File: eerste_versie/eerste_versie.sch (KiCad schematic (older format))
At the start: 16 parts, among them U1 ESP32-WROOM-32U, U2 AMS1117-3.3, X1 DG3XX-02-5.0

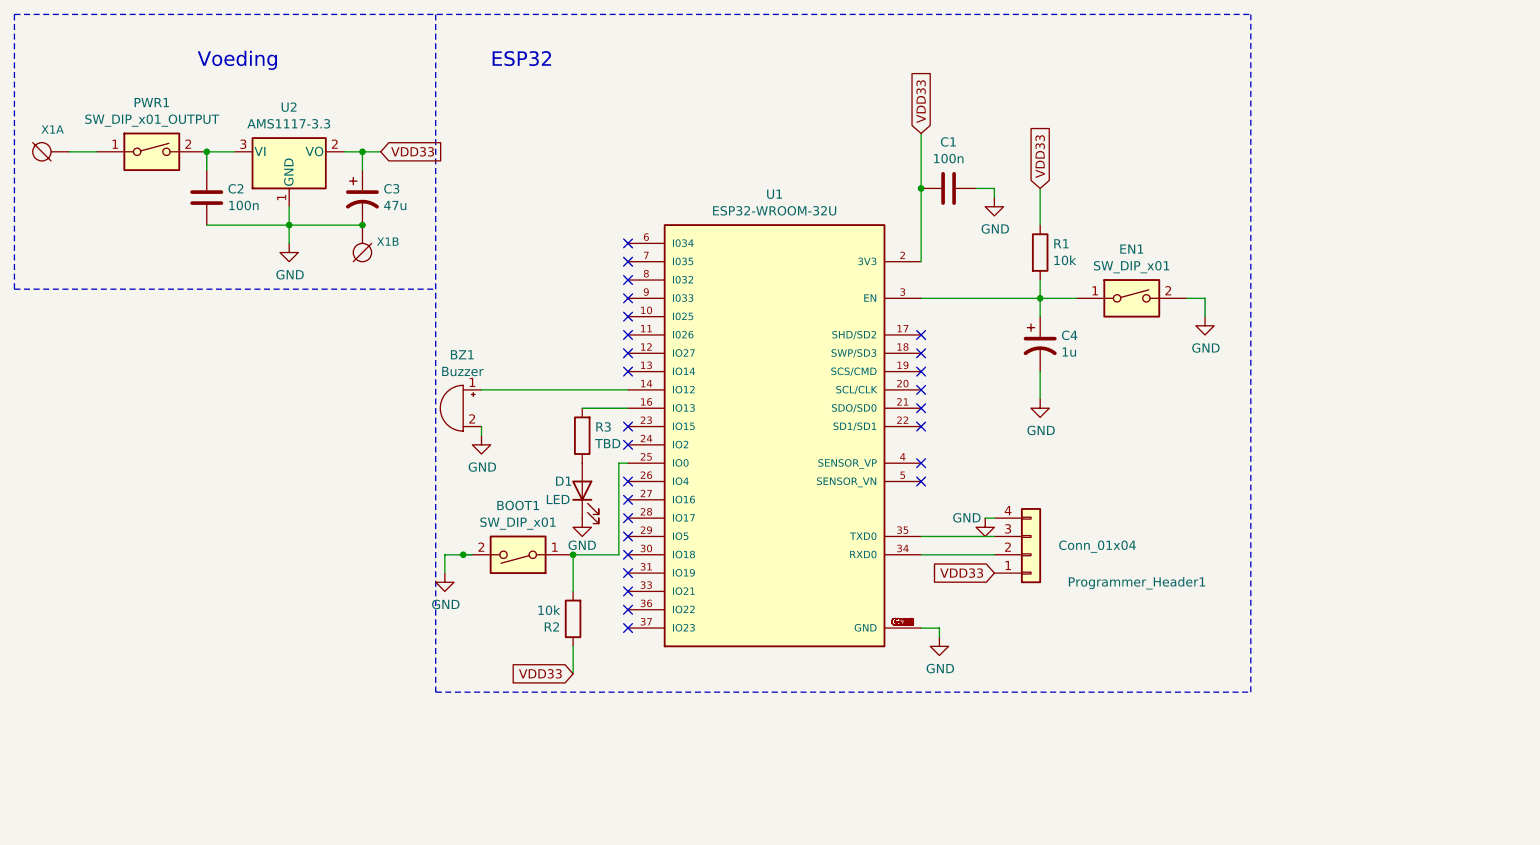
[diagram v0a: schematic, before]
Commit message: volledige versie
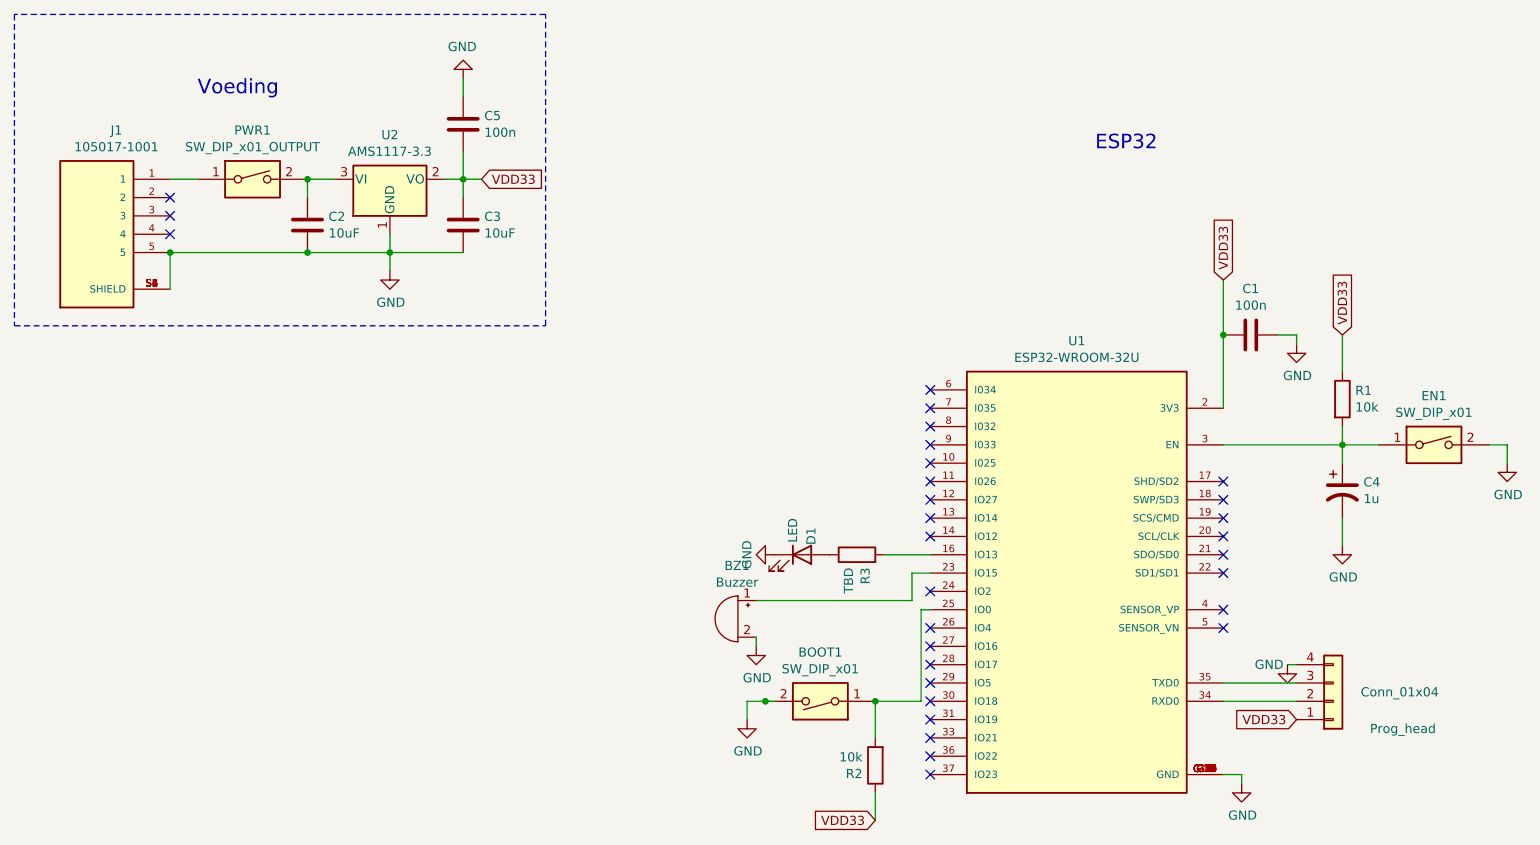
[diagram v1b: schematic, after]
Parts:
- removed C3: 47u, Capacitor_SMD:CP_Elec_6.3x3, symbol Device:CP1
- removed X1: DG3XX-02-5.0, degson:degson-DG306-5.0-02P, symbol eerste_versie-rescue:DG3XX-02-5.0-degson
- added C3: 10uF, Capacitor_SMD:C_0805_2012Metric_Pad1.18x1.45mm_HandSolder, symbol Device:C
- added C5: 100n, Capacitor_SMD:C_0805_2012Metric_Pad1.18x1.45mm_HandSolder, symbol Device:C
- added J1: 105017-1001, 105017-1001:MOLEX_105017-1001, symbol 105017-1001:105017-1001
- BOOT1, EN1: footprint Button_Switch_SMD:SW_SPST_B3U-1000P -> 434111043826:434111043826
- C2: value 100n -> 10uF
- PWR1: footprint Button_Switch_SMD:SW_DIP_SPSTx01_Slide_6.7x4.1mm_W6.73mm_P2.54mm_LowProfile_JPin -> sparkfun:SWITCH_SPST_SMD_A
- Prog_head: renamed from Programmer_Header1; footprint Connector_PinHeader_2.00mm:PinHeader_1x04_P2.00mm_Vertical -> Connector_PinHeader_2.54mm:PinHeader_1x04_P2.54mm_Vertical
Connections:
- net GND: now also C3.2, C5.1, J1.5, J1.S1 (SHIELD), J1.S2 (SHIELD), J1.S3 (SHIELD), J1.S4 (SHIELD), J1.S5 (SHIELD), J1.S6 (SHIELD)
- net VDD33: now also C3.1, C5.2
- net at U1.14 (IO12): no longer BZ1.1 (-)
- net at U1.23 (IO15): now also BZ1.1 (-)
- net at PWR1.1: now also J1.1
- no-connect marks 27 -> 30
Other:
- moved on the sheet: BOOT1, BZ1, C1, C2, C4, D1, EN1, PWR1, Prog_head, R1, R2, R3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
